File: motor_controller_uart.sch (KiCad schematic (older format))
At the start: 34 parts, among them J10 DB9_Male, J11 DB9_Male, J8 DB9_Male, J9 DB9_Male, U2 MAX3232, U4 MAX3232

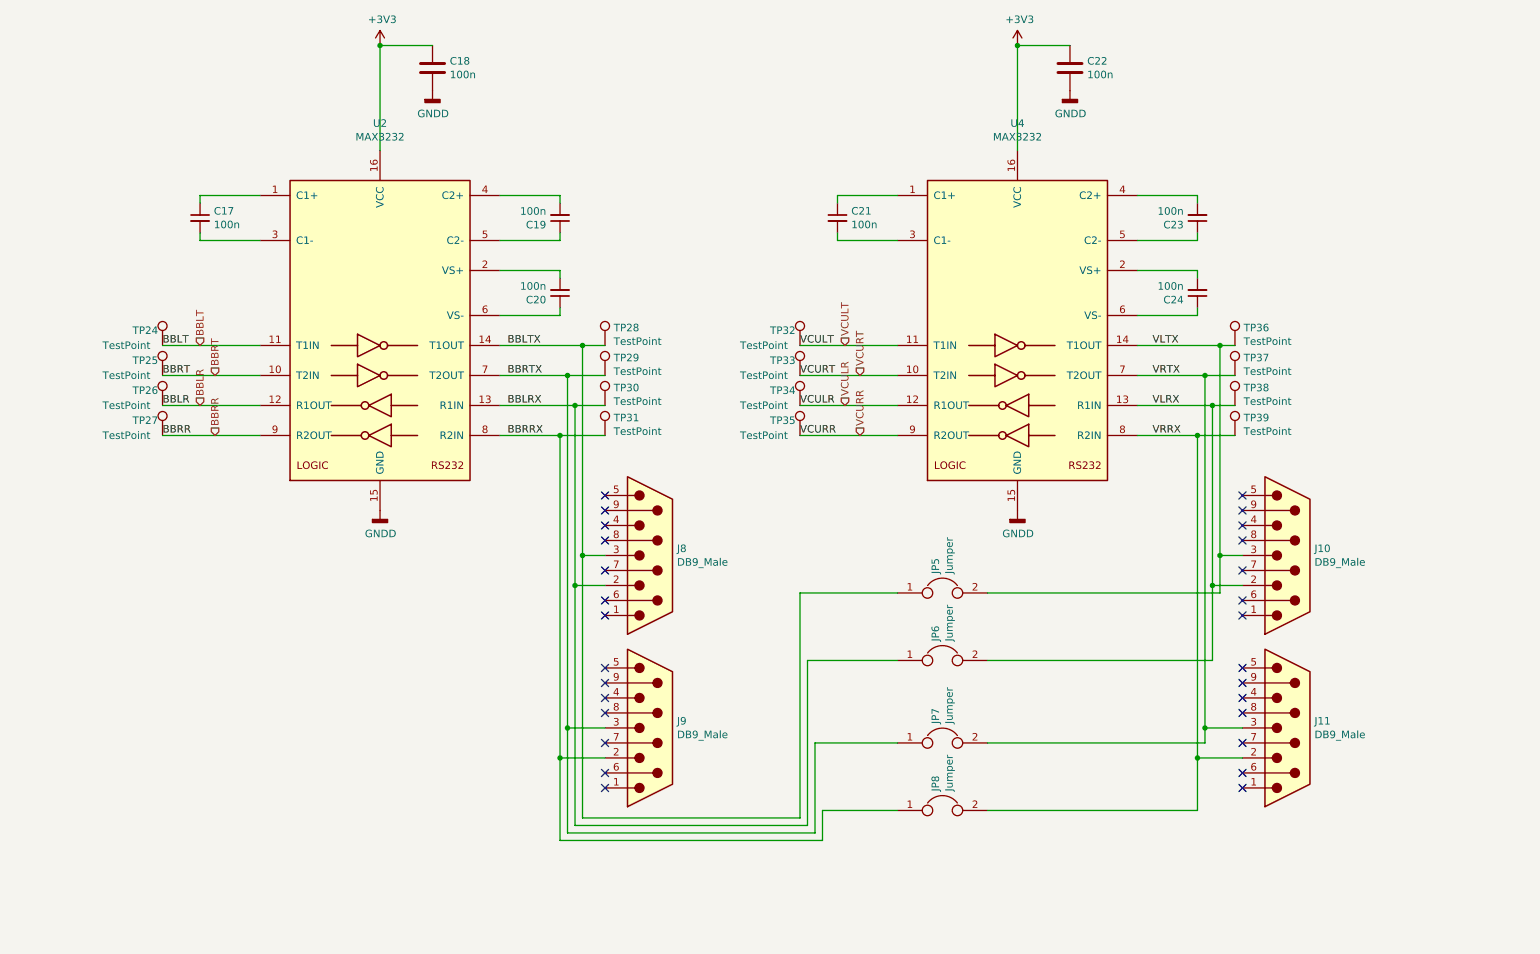
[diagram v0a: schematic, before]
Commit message: new, compact (and sexy) design
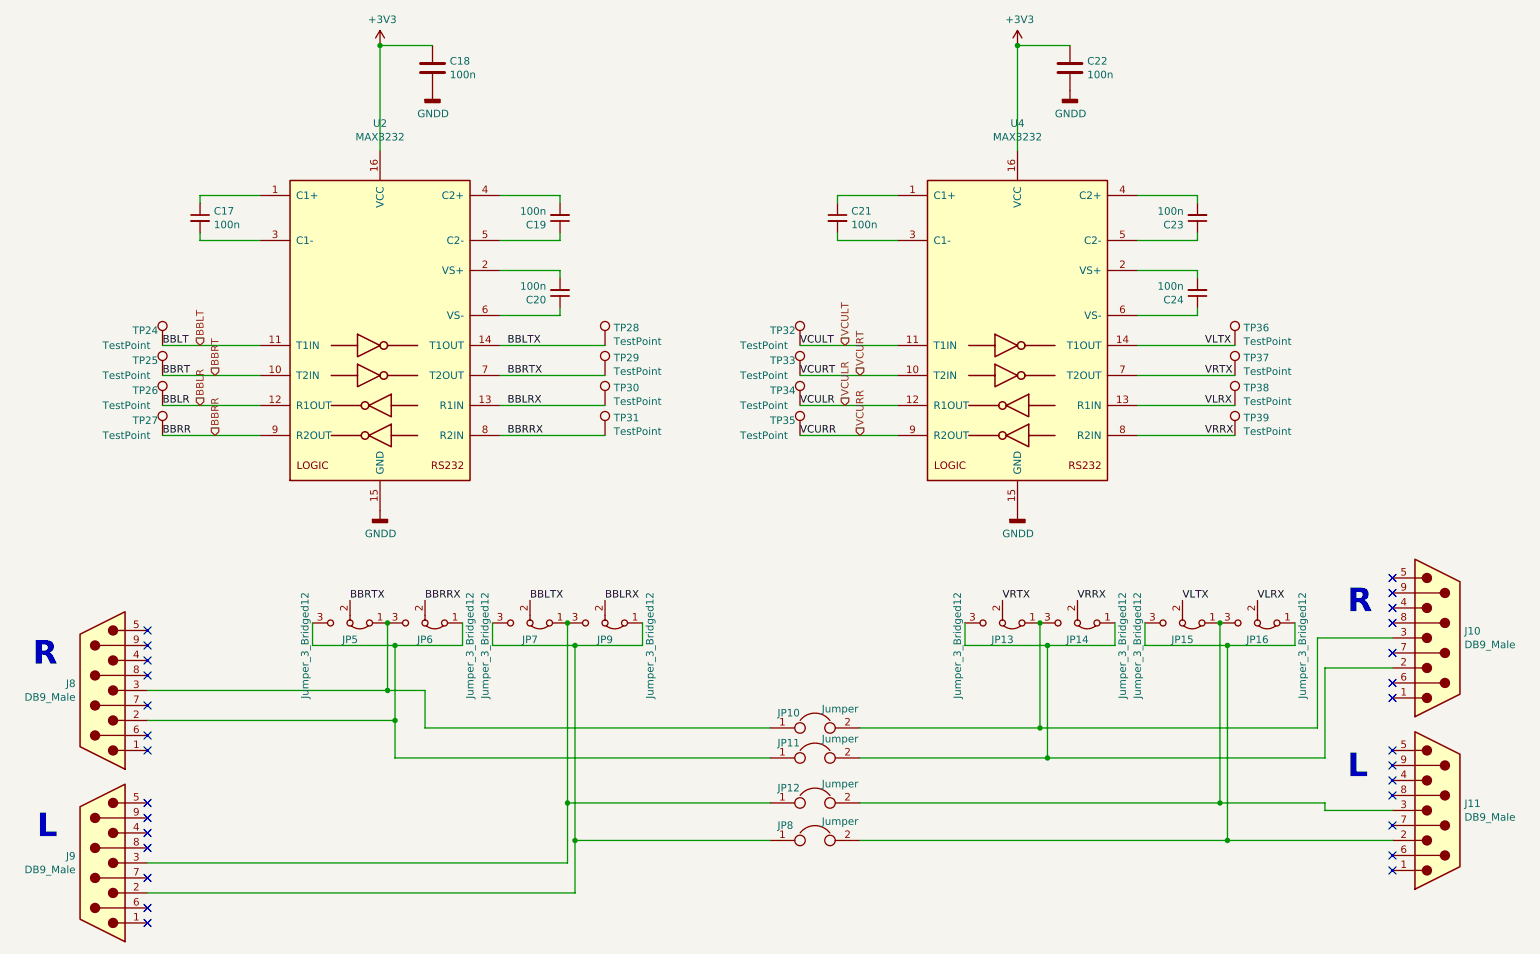
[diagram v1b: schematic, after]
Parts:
- removed JP5, JP6, JP7: Jumper, Connector_PinHeader_2.00mm:PinHeader_1x03_P2.00mm_Vertical, symbol Device:Jumper
- added JP10, JP11, JP12: Jumper, Connector_PinHeader_2.00mm:PinHeader_1x03_P2.00mm_Vertical, symbol Device:Jumper
- added JP13, JP14, JP15, JP16, JP5, JP6, JP7, JP9: Jumper_3_Bridged12, Connector_PinHeader_2.00mm:PinHeader_1x03_P2.00mm_Vertical, symbol Jumper:Jumper_3_Bridged12
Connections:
- net BBLRX: now also JP9.2 (C); no longer J8.2
- net BBLTX: now also JP7.2 (C); no longer J8.3
- net BBRRX: now also JP6.2 (C); no longer J9.2, JP8.1
- net BBRTX: now also JP5.2 (C); no longer J9.3
- net VLRX: now also JP16.2 (C); no longer J10.2
- net VLTX: now also JP15.2 (C); no longer J10.3
- net VRRX: now also JP14.2 (C); no longer J11.2, JP8.2
- net VRTX: now also JP13.2 (C); no longer J11.3
- new net: J9.3, JP12.1, JP7.1 (A), JP9.3 (B)
- new net: J9.2, JP7.3 (B), JP8.1, JP9.1 (A)
- new net: J8.3, JP10.1, JP5.1 (A), JP6.3 (B)
- new net: J8.2, JP11.1, JP5.3 (B), JP6.1 (A)
- new net: J11.3, JP12.2, JP15.1 (A), JP16.3 (B)
- new net: J11.2, JP15.3 (B), JP16.1 (A), JP8.2
- new net: J10.3, JP10.2, JP13.1 (A), JP14.3 (B)
- new net: J10.2, JP11.2, JP13.3 (B), JP14.1 (A)
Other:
- note added: "L"
- note added: "R"
- moved on the sheet: J10, J11, J8, J9, JP8

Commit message: forgot to save schematic
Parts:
- J10, J11, J8, J9: footprint Connector_Dsub:DSUB-9_Male_Horizontal_P2.77x2.84mm_EdgePinOffset7.70mm_Housed_MountingHolesOffset9.12mm -> Connector_Dsub:DSUB-9_Male_Vertical_P2.77x2.84mm_MountingHoles
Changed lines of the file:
@@
 F 0 "J8" H 1780 5196 50  0000 L CNN
 F 1 "DB9_Male" H 1780 5105 50  0000 L CNN
-F 2 "Connector_Dsub:DSUB-9_Male_Horizontal_P2.77x2.84mm_EdgePinOffset7.70mm_Housed_MountingHolesOffset9.12mm" H 1600 5150 50  0001 C CNN
+F 2 "Connector_Dsub:DSUB-9_Male_Vertical_P2.77x2.84mm_MountingHoles" H 1600 5150 50  0001 C CNN
 F 3 " ~" H 1600 5150 50  0001 C CNN
 F 4 "5747840-3" H 1600 5150 50  0001 C CNN "Part"
@@
 F 0 "J9" H 1780 6346 50  0000 L CNN
 F 1 "DB9_Male" H 1780 6255 50  0000 L CNN
-F 2 "Connector_Dsub:DSUB-9_Male_Horizontal_P2.77x2.84mm_EdgePinOffset7.70mm_Housed_MountingHolesOffset9.12mm" H 1600 6300 50  0001 C CNN
+F 2 "Connector_Dsub:DSUB-9_Male_Vertical_P2.77x2.84mm_MountingHoles" H 1600 6300 50  0001 C CNN
 F 3 " ~" H 1600 6300 50  0001 C CNN
 F 4 "5747840-3" H 1600 6300 50  0001 C CNN "Part"
@@
 F 0 "J10" H 10680 4846 50  0000 L CNN
 F 1 "DB9_Male" H 10680 4755 50  0000 L CNN
-F 2 "Connector_Dsub:DSUB-9_Male_Horizontal_P2.77x2.84mm_EdgePinOffset7.70mm_Housed_MountingHolesOffset9.12mm" H 10500 4800 50  0001 C CNN
+F 2 "Connector_Dsub:DSUB-9_Male_Vertical_P2.77x2.84mm_MountingHoles" H 10500 4800 50  0001 C CNN
 F 3 " ~" H 10500 4800 50  0001 C CNN
 F 4 "5747840-3" H 10500 4800 50  0001 C CNN "Part"
@@
 F 0 "J11" H 10680 5996 50  0000 L CNN
 F 1 "DB9_Male" H 10680 5905 50  0000 L CNN
-F 2 "Connector_Dsub:DSUB-9_Male_Horizontal_P2.77x2.84mm_EdgePinOffset7.70mm_Housed_MountingHolesOffset9.12mm" H 10500 5950 50  0001 C CNN
+F 2 "Connector_Dsub:DSUB-9_Male_Vertical_P2.77x2.84mm_MountingHoles" H 10500 5950 50  0001 C CNN
 F 3 " ~" H 10500 5950 50  0001 C CNN
 F 4 "5747840-3" H 10500 5950 50  0001 C CNN "Part"
